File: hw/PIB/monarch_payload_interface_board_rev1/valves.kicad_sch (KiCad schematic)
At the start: 4 parts, among them U3 NZT7053

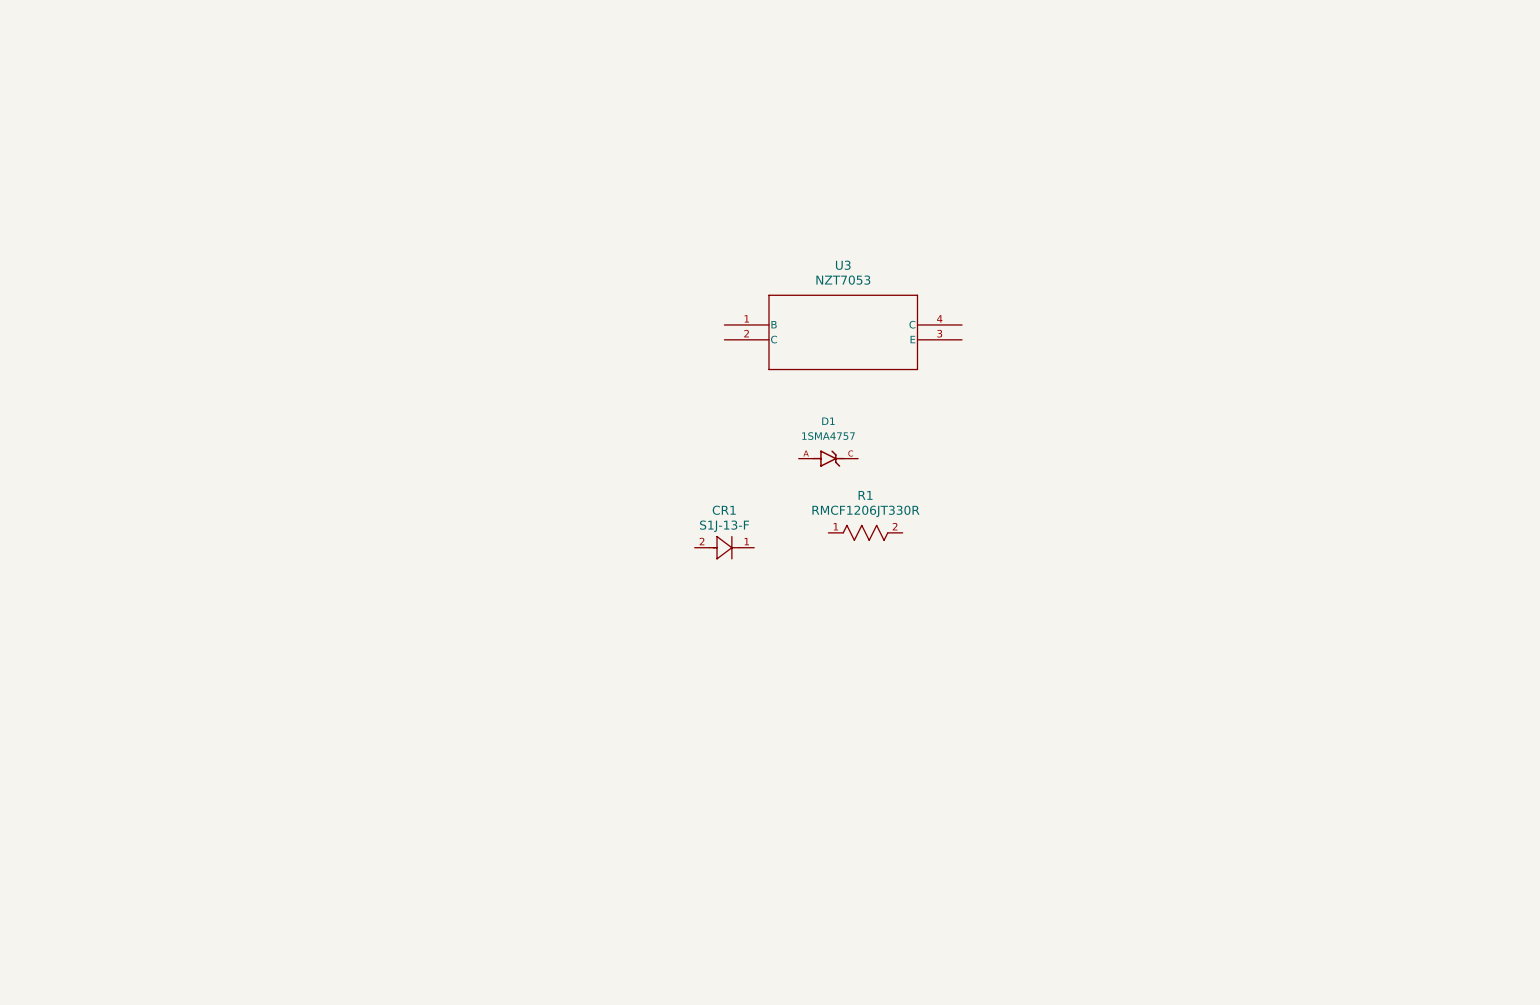
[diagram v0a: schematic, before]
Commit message: More components
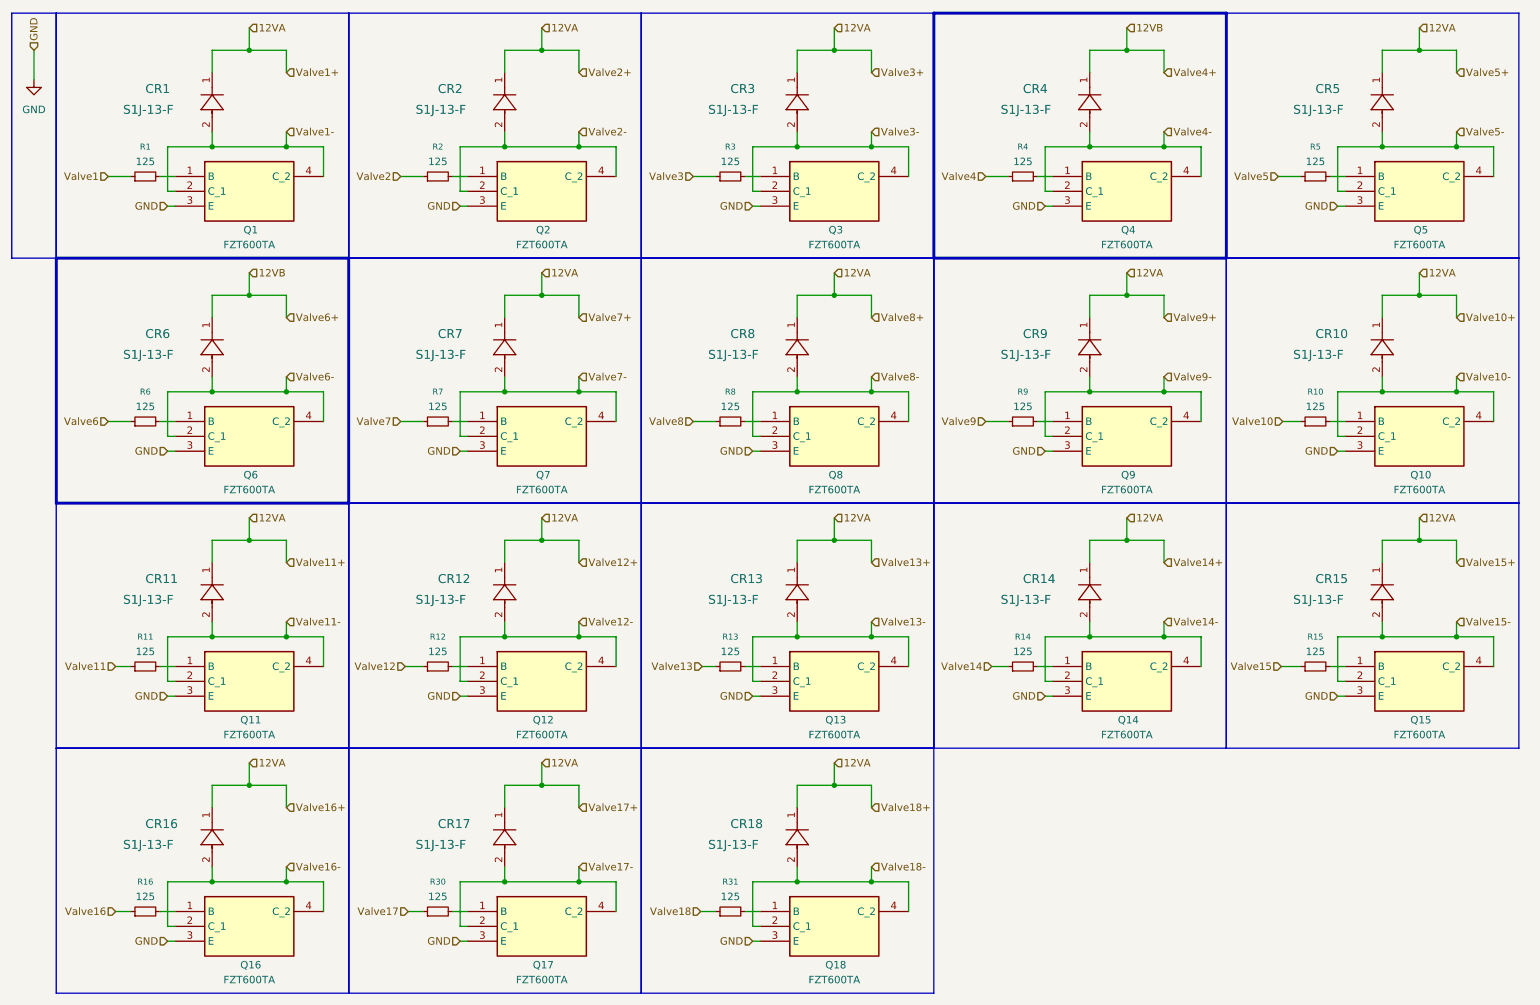
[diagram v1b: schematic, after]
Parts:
- removed D1: 1SMA4757, Zener_diode:DIOM4325X250N, symbol 1SMA4757:1SMA4757
- removed R1: RMCF1206JT330R, 330O res:STA_RMCF1206_STP-L, symbol 330O res:RMCF1206JT330R
- removed U3: NZT7053, nzt7:SOT-223_ONS-L, symbol nzt7:NZT7053
- added CR10, CR11, CR12, CR13, CR14, CR15, CR16, CR17, CR18, CR2, CR3, CR4, CR5, CR6, CR7, CR8, CR9: S1J-13-F, s1j:SMA_DIO-L, symbol s1j:S1J-13-F
- added Q1, Q10, Q11, Q12, Q13, Q14, Q15, Q16, Q17, Q18, Q2, Q3, Q4, Q5, Q6, Q7, Q8, Q9: FZT600TA, fzt:SOT230P700X170-4N, symbol FZT600TA:FZT600TA
- added R1, R10, R11, R12, R13, R14, R15, R16, R2, R3, R30, R31, R4, R5, R6, R7, R8, R9: 125, Resistor_SMD:R_0402_1005Metric, symbol Device:R_Small
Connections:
- net 12VA: now reaches CR1.1
- net 12VA: now also CR10.1, CR11.1, CR12.1, CR13.1, CR14.1, CR15.1, CR16.1, CR17.1, CR18.1, CR2.1, CR3.1, CR5.1, CR7.1, CR8.1, CR9.1
- net Valve1-: now reaches CR1.2
- net Valve1-: now also Q1.2 (C_1), Q1.4 (C_2)
- new net: Q3.1 (B), R3.2
- new net: Q6.1 (B), R6.2
- new net: Q5.1 (B), R5.2
- new net: Q15.1 (B), R15.2
- new net: Q8.1 (B), R8.2
- new net: Q12.1 (B), R12.2
- new net: Q7.1 (B), R7.2
- new net: Q13.1 (B), R13.2
- new net: Q14.1 (B), R14.2
- new net: Q4.1 (B), R4.2
- new net: Q17.1 (B), R30.2
- new net: Q16.1 (B), R16.2
- new net: Q2.1 (B), R2.2
- new net: Q10.1 (B), R10.2
- new net: Q1.1 (B), R1.2
- new net: Q18.1 (B), R31.2
- new net: Q9.1 (B), R9.2
- new net: Q11.1 (B), R11.2
- new net 12VB: CR4.1, CR6.1
- new net GND: Q1.3 (E), Q10.3 (E), Q11.3 (E), Q12.3 (E), Q13.3 (E), Q14.3 (E), Q15.3 (E), Q16.3 (E), Q17.3 (E), Q18.3 (E), Q2.3 (E), Q3.3 (E), Q4.3 (E), Q5.3 (E), Q6.3 (E), Q7.3 (E), Q8.3 (E), Q9.3 (E)
- new net Valve1: R1.1
- new net Valve10: R10.1
- new net Valve10-: CR10.2, Q10.2 (C_1), Q10.4 (C_2)
- new net Valve11: R11.1
- new net Valve11-: CR11.2, Q11.2 (C_1), Q11.4 (C_2)
- new net Valve12: R12.1
- new net Valve12-: CR12.2, Q12.2 (C_1), Q12.4 (C_2)
- new net Valve13: R13.1
- new net Valve13-: CR13.2, Q13.2 (C_1), Q13.4 (C_2)
- new net Valve14: R14.1
- new net Valve14-: CR14.2, Q14.2 (C_1), Q14.4 (C_2)
- new net Valve15: R15.1
- new net Valve15-: CR15.2, Q15.2 (C_1), Q15.4 (C_2)
- new net Valve16: R16.1
- new net Valve16-: CR16.2, Q16.2 (C_1), Q16.4 (C_2)
- new net Valve17: R30.1
- new net Valve17-: CR17.2, Q17.2 (C_1), Q17.4 (C_2)
- new net Valve18: R31.1
- new net Valve18-: CR18.2, Q18.2 (C_1), Q18.4 (C_2)
- new net Valve2: R2.1
- new net Valve2-: CR2.2, Q2.2 (C_1), Q2.4 (C_2)
- new net Valve3: R3.1
- new net Valve3-: CR3.2, Q3.2 (C_1), Q3.4 (C_2)
- new net Valve4: R4.1
- new net Valve4-: CR4.2, Q4.2 (C_1), Q4.4 (C_2)
- new net Valve5: R5.1
- new net Valve5-: CR5.2, Q5.2 (C_1), Q5.4 (C_2)
- new net Valve6: R6.1
- new net Valve6-: CR6.2, Q6.2 (C_1), Q6.4 (C_2)
- new net Valve7: R7.1
- new net Valve7-: CR7.2, Q7.2 (C_1), Q7.4 (C_2)
- new net Valve8: R8.1
- new net Valve8-: CR8.2, Q8.2 (C_1), Q8.4 (C_2)
- new net Valve9: R9.1
- new net Valve9-: CR9.2, Q9.2 (C_1), Q9.4 (C_2)
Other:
- moved on the sheet: CR1
